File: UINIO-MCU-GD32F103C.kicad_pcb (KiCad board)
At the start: 2 copper layers, 67.4 x 20.3 mm, 43 parts, among them J1 Conn_01x24_Male, J2 Conn_01x24_Male, J3 Conn_01x04_Male, SW1 BOOT1, SW2 NRST, SW3 BOOT0, U1 ME6211C33M5G-N, U2 GD32F103C8T6, Y1 32.768KHz, Y2 8MHz

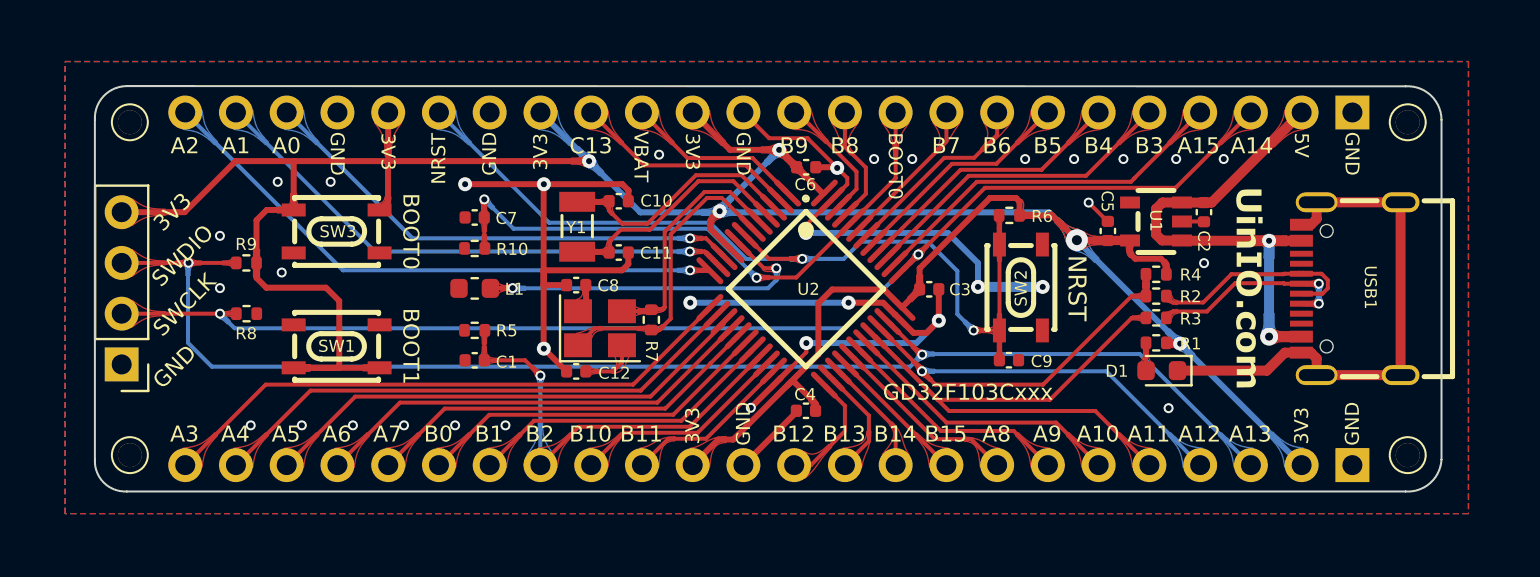
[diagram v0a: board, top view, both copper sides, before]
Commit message: Prepare version 2.0.0.
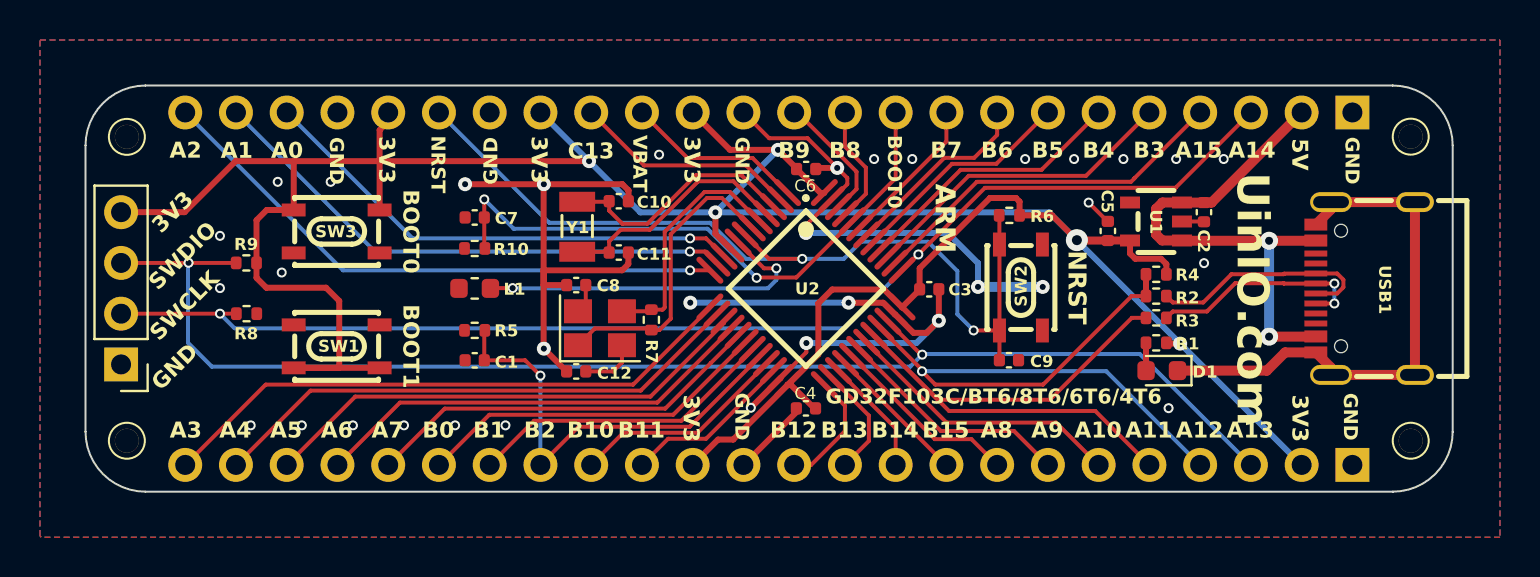
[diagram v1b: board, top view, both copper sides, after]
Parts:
- removed the ? at (177.3, 100.7)
- removed the ? at (166.1, 100.9)
- removed the ? at (143.6, 100.7)
- removed the ? at (171.9, 100.9)
- added ?: LOGO, LOGO, B.Cu at (167.8, 100.7)
- added ?: LOGO, LOGO, B.Cu at (140.6, 100.7)
- J1, J2: value Conn_01x24_Male -> Conn_01x24_Pin
- J3: value Conn_01x04_Male -> Conn_01x04_Pin
- moved HOLE** 0.75 mm to (121.1, 93.1)
- moved HOLE** 0.74 mm to (185.3, 108.3)
- moved HOLE** 0.74 mm to (185.3, 93.1)
- moved HOLE** 0.74 mm to (121.1, 108.3)
- moved USB1 0.72 mm to (183.1, 100.7)
- moved C4 0.12 mm to (155.1, 106.7)
- moved C6 0.09 mm to (155.1, 94.7)
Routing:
- net /VDD_5V: track 24.3 -> 25.8 mm
- net /VDD_3.3V: track 149.7 -> 148.6 mm
- net /USB_Data-: track 10.2 -> 11.1 mm
- net /USB_Data+: track 10.8 -> 11.6 mm
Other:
- board size 67.4 x 20.3 mm -> 68.4 x 20.3 mm
- board text added: "ARM"
- board text added: "GD32F103C/BT6/8T6/6T6/4T6"
- board text added: "UinIO.com"
- board text added: "Version 2.0.0"
- board text removed: "GD32F103Cxxx"
- board text removed: "Version 1.0.0"
